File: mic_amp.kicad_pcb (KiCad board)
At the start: 2 copper layers, 47 x 29 mm, 25 parts

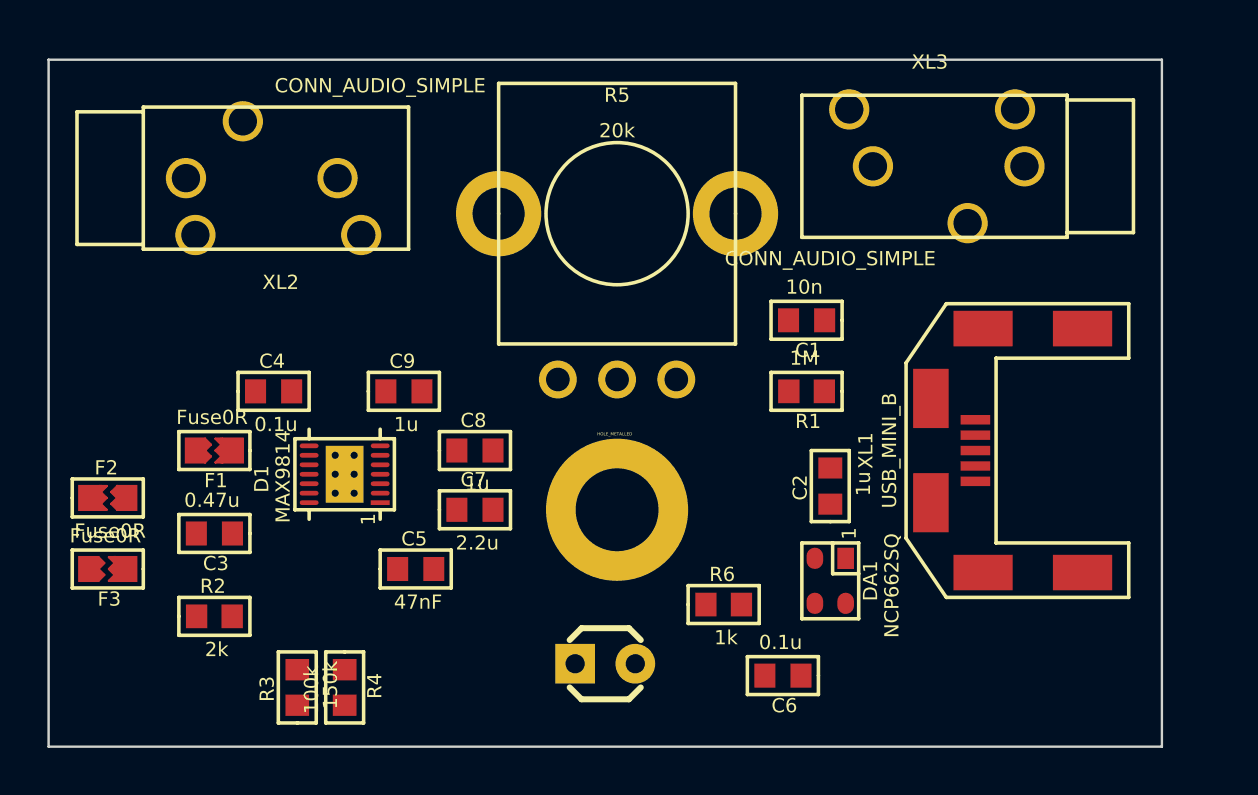
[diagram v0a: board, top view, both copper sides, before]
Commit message: filling wanted :)
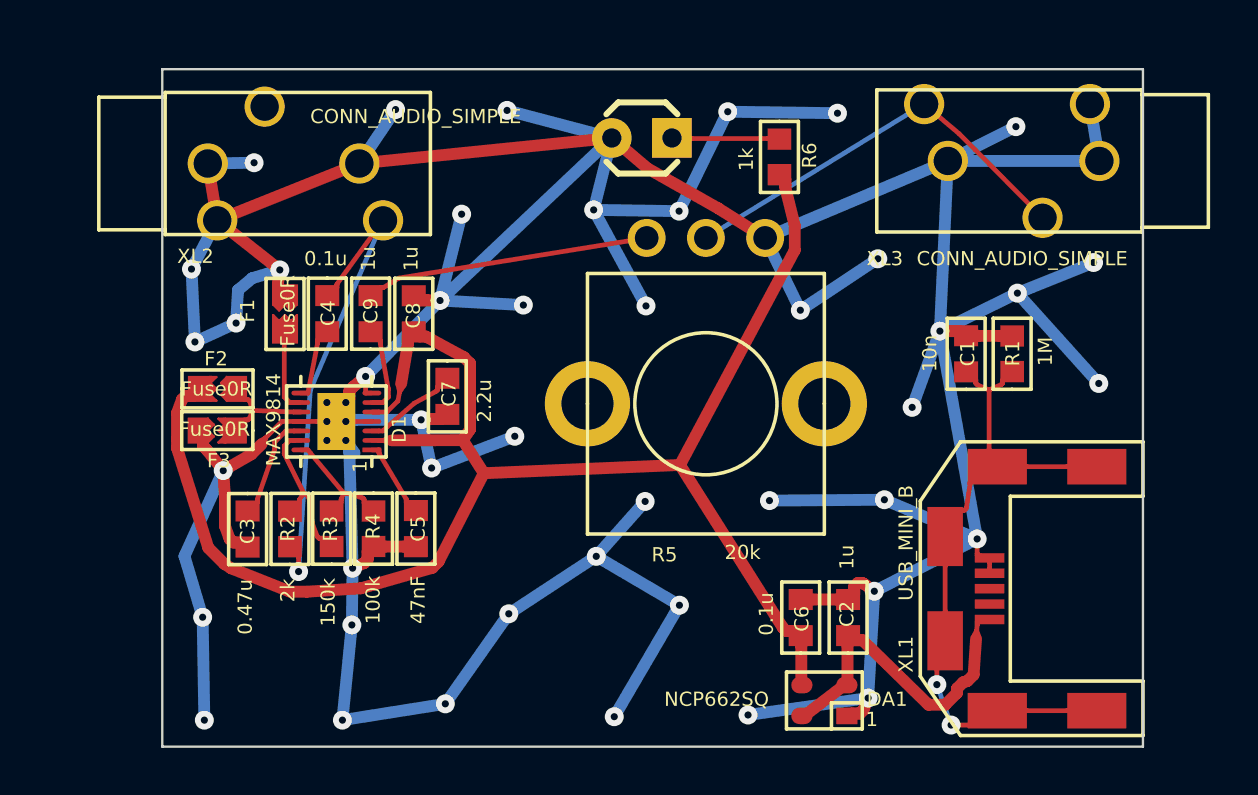
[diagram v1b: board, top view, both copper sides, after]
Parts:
- removed HOLE1: HOLE_METALLED, PCB:Hole3_5_out6mm
- moved D2 22.2 mm to (210.0, 91.3), turned to 180 degrees
- moved R6 19.0 mm to (215.9, 92.1), turned to 270 degrees
- moved R5 8.86 mm to (212.8, 102.5), turned to 180 degrees
- moved R1 8.82 mm to (225.7, 100.4), turned to 90 degrees
- moved F3 7.45 mm to (192.1, 103.7)
- moved C1 6.88 mm to (223.7, 100.4), turned to 90 degrees
- moved R3 6.86 mm to (197.0, 107.8)
- moved R4 6.81 mm to (198.7, 107.8)
- moved F2 6.53 mm to (192.1, 101.9)
- moved F1 6.49 mm to (195.0, 98.7), turned to 90 degrees
- moved C8 6.32 mm to (200.4, 98.7), turned to 90 degrees
- moved XL1 5.86 mm to (225.6, 110.3)
- moved C2 5.60 mm to (218.8, 111.6)
- moved DA1 5.06 mm to (217.8, 115.1), turned to 180 degrees
- moved C7 4.93 mm to (201.8, 102.2), turned to 270 degrees
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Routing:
- net GND: track 0.00 -> 266.6 mm, vias 0 -> 45
- net VDD: track 0.00 -> 72.4 mm
- net Net-(C1-Pad1): track 0.00 -> 28.6 mm, vias 0 -> 2
- net Net-(C4-Pad1): track 0.00 -> 20.7 mm, vias 0 -> 1
- net Net-(R5-Pad3): track 0.00 -> 17.7 mm
- net Net-(C2-Pad1): track 0.00 -> 15.0 mm
- net Net-(C9-Pad2): track 0.00 -> 12.0 mm
- net /MICBIAS: track 0.00 -> 6.73 mm
- net Net-(D1-Pad14): track 0.00 -> 5.21 mm
- net Net-(D2-PadA): track 0.00 -> 4.54 mm
- net Net-(C3-Pad1): track 0.00 -> 4.52 mm
- net Net-(D1-Pad10): track 0.00 -> 4.45 mm
- net Net-(C7-Pad1): track 0.00 -> 4.05 mm
- net Net-(C9-Pad1): track 0.00 -> 3.77 mm
- net Net-(D1-Pad9): track 0.00 -> 3.55 mm
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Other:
- board size 47 x 29 mm -> 41.4 x 28.6 mm
